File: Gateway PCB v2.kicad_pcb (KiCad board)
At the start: 4 copper layers, 83.6 x 39.8 mm, 114 parts, among them J1 Conn_Coaxial, J2 Conn_01x04_Pin, J3 Conn_02x03_Odd_Even, J4 Conn_01x03_Pin, U6 TPS7A91, U7 TLV62568ADRL, X1 TG2016SMN 32.0000M-TCGNNMB

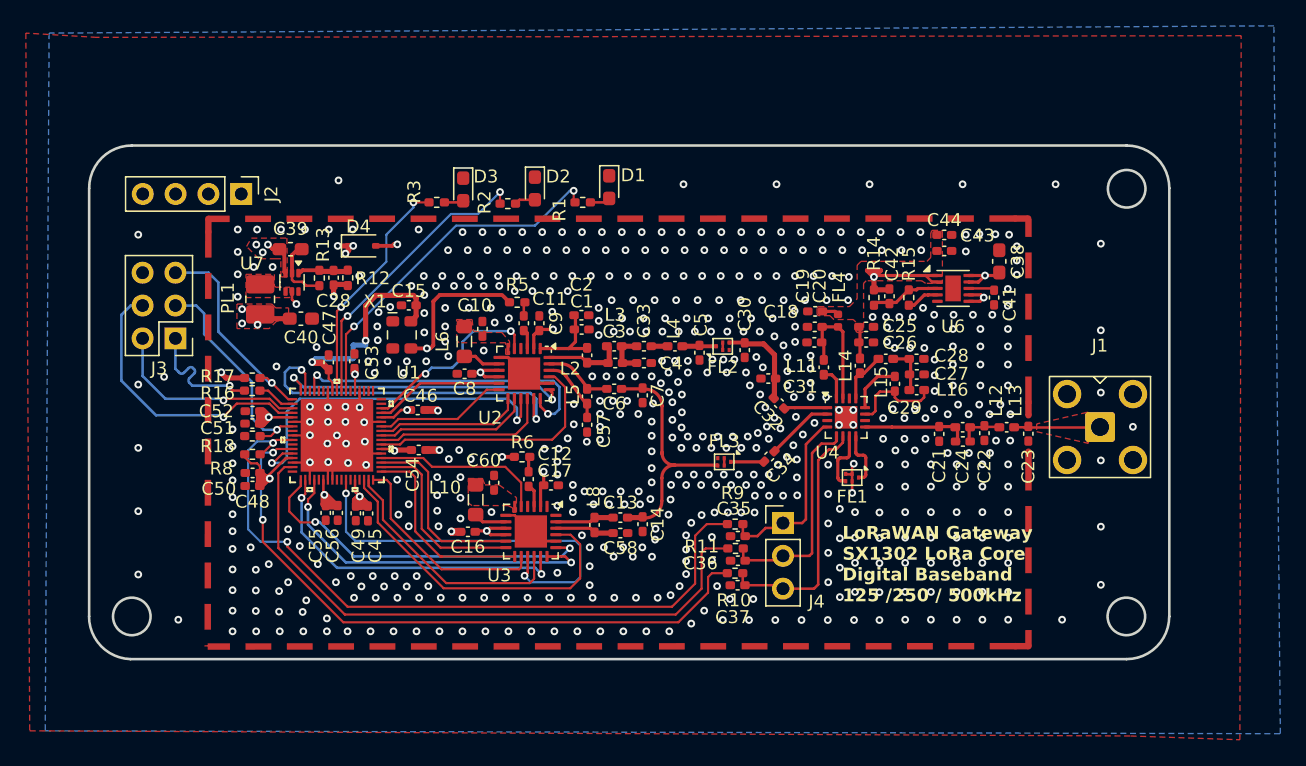
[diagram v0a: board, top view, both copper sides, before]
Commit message: Increse size
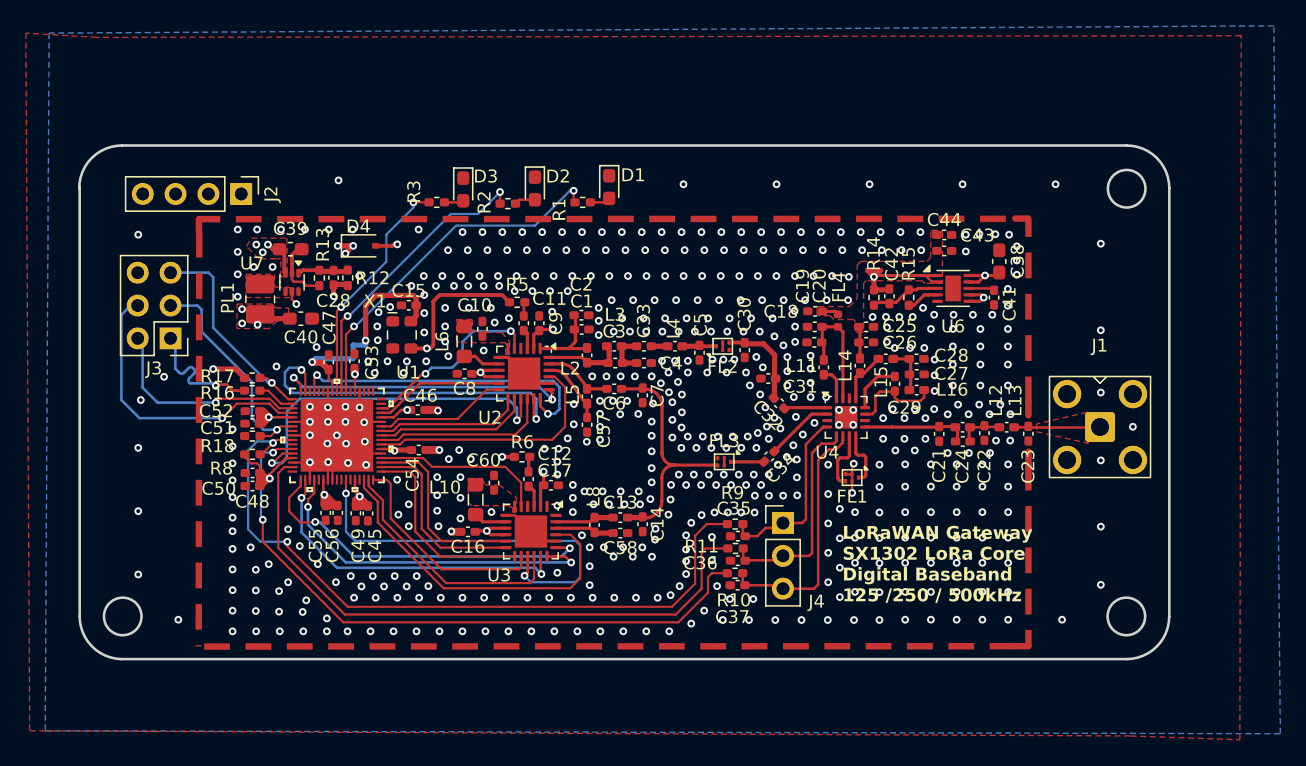
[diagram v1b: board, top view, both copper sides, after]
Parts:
- moved NT4 0.73 mm to (22.3, 70.9)
- moved J3 0.38 mm to (20.1, 79.6)
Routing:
- net 3.3V: track 98.0 -> 134.6 mm
- net EX_HOST_SCK: track 22.2 -> 23.4 mm
- net EX_HOST_MOSI: track 15.7 -> 16.3 mm
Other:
- board size 83.6 x 39.8 mm -> 84.4 x 39.8 mm
